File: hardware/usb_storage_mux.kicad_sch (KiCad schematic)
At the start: 25 parts, among them J8 Hirose USB3_B_Micro, J9 USB3_A, U6 TMUXHS4212

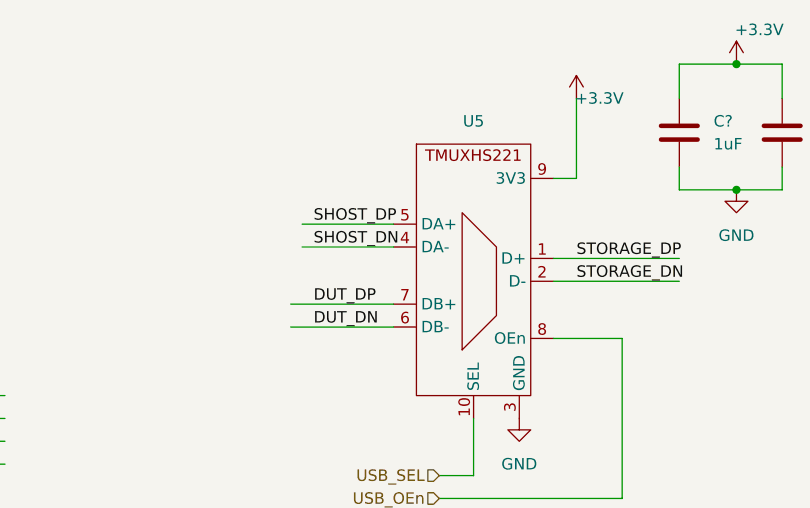
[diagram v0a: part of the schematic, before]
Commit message: Almost ready 2.0.0
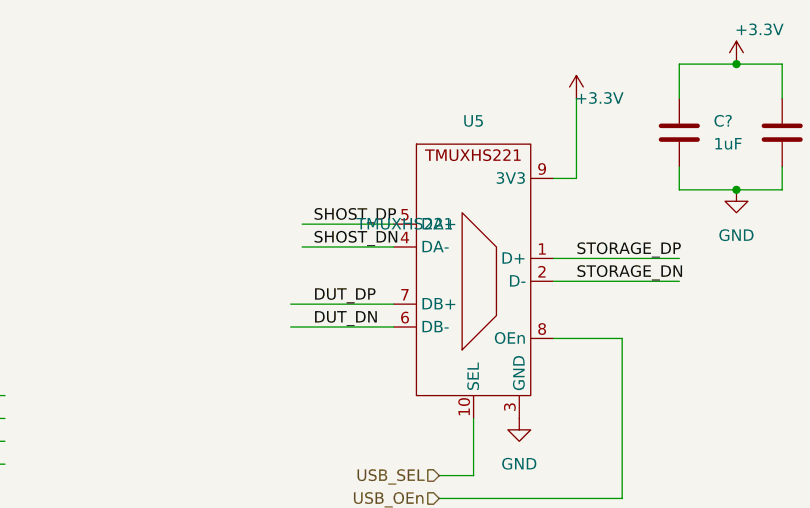
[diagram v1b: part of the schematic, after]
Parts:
- C25, C26, C27, C28, C? (x4): MFN (none) -> CL10B104KB8NNNC
- C? (x2): footprint Capacitor_SMD:C_0402_1005Metric -> Capacitor_SMD:C_0603_1608Metric; MFN (none) -> CL10B105KA8NNNC; MPN (none) -> CL10B105KA8NNNC
- C?: MFN (none) -> HV470M035E055ETR; MPN (none) -> HV470M035E055ETR
- D8: Link (none) -> https://www2.mouser.com/ProductDetail/onsemi-Fairchild/1N44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; MFN (none) -> 1N4448WT; MPN (none) -> 1N4448WT
- F2: MFN (none) -> MF-MSMF125-2; MPN (none) -> MF-MSMF125-2
- J8: Link https://www.mouser.es/c/connectors/usb-connectors/?product=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 -> https://www2.mouser.com/ProductDetail/Hirose-Connector/ZX36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; MFN (none) -> ZX360D-B-10P(30)
- J9: Link (none) -> https://eu.mouser.com/ProductDetail/Molex/48393-0001?qs=4Ef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; MFN (none) -> 48393-0001; MPN (none) -> 48393-0001
- Q? (x2): Link (none) -> https://www.mouser.es/ProductDetail/onsemi-Fairchild/FDC633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; MFN (none) -> FDC6330L; MPN (none) -> FDC6330L
- R? (x2): MFN (none) -> RTT024702FTH; MPN (none) -> RTT024702FTH
- R? (x2): MFN (none) -> RTT022201FTH; MPN (none) -> RTT022201FTH
- R? (x2): MFN (none) -> RTT02331JTH; MPN (none) -> RTT02331JTH
- U5: value ~ -> TMUXHS221; Link (none) -> https://eu.mouser.com/ProductDetail/Texas-Instruments/TMUXH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; MFN (none) -> TMUXHS221NKGR; MPN (none) -> TMUXHS221NKGR
- U6: Link (none) -> https://eu.mouser.com/ProductDetail/Texas-Instruments/TMUXH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; MFN (none) -> TMUXHS4212RKSR; MPN (none) -> TMUXHS4212RKSR
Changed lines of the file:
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@@
+      (effects (font (size 1.27 1.27)) hide)
+    )
+    (property "MFN" "RTT024702FTH" (at 195.58 85.09 0)
+      (effects (font (size 1.27 1.27)) hide)
+    )
+    (property "MPN" "RTT024702FTH" (at 195.58 85.09 0)
       (effects (font (size 1.27 1.27)) hide)
     )
@@
       (effects (font (size 1.27 1.27)) hide)
     )
+    (property "MFN" "CL10B104KB8NNNC" (at 163.83 113.03 0)
+      (effects (font (size 1.27 1.27)) hide)
+    )
     (pin "1")
     (pin "2")
@@
     )
     (property "Datasheet" "https://www.onsemi.com/pub/Collateral/FDC6330L-D.PDF" (at 207.01 90.17 0)
+      (effects (font (size 1.27 1.27)) hide)
+    )
+    (property "Link" "https://www.mouser.es/ProductDetail/onsemi-Fairchild/FDC6330L?qs=efMQ9B2bthfkfJJoj5%252B07g%3D%3D" (at 209.55 87.63 0)
+      (effects (font (size 1.27 1.27)) hide)
+    )
+    (property "MFN" "FDC6330L" (at 209.55 87.63 0)
+      (effects (font (size 1.27 1.27)) hide)
+    )
+    (property "MPN" "FDC6330L" (at 209.55 87.63 0)
       (effects (font (size 1.27 1.27)) hide)
     )
@@
       (effects (font (size 1.27 1.27)) hide)
     )
-    (property "Link" "https://www.mouser.es/c/connectors/usb-connectors/?product=Micro%20USB%20Type%20B%20Connectors&standard=USB%203.0&termination%20style=SMD%2FSMT&instock=y" (at 31.75 154.94 0)
+    (property "Link" "https://www2.mouser.com/ProductDetail/Hirose-Connector/ZX360D-B-10P30?qs=4J5DPWWS9EDezzYtx6NKEg%3D%3D" (at 31.75 154.94 0)
+      (effects (font (size 1.27 1.27)) hide)
+    )
+    (property "MFN" "ZX360D-B-10P(30)" (at 31.75 154.94 0)
       (effects (font (size 1.27 1.27)) hide)
     )
@@
       (effects (font (size 1.27 1.27)) hide)
     )
+    (property "MFN" "CL10B104KB8NNNC" (at 26.67 186.055 0)
+      (effects (font (size 1.27 1.27)) hide)
+    )
     (pin "1")
     (pin "2")
@@
       (effects (font (size 1.27 1.27)) (justify left))
     )
-    (property "Footprint" "Capacitor_SMD:C_0402_1005Metric" (at 158.4452 146.05 0)
+    (property "Footprint" "Capacitor_SMD:C_0603_1608Metric" (at 158.4452 146.05 0)
       (effects (font (size 1.27 1.27)) hide)
     )
@@
       (effects (font (size 1.27 1.27)) hide)
     )
+    (property "MFN" "CL10B105KA8NNNC" (at 157.48 142.24 0)
+      (effects (font (size 1.27 1.27)) hide)
+    )
+    (property "MPN" "CL10B105KA8NNNC" (at 157.48 142.24 0)
+      (effects (font (size 1.27 1.27)) hide)
+    )
     (pin "1")
     (pin "2")
@@
       (effects (font (size 1.27 1.27)) hide)
     )
+    (property "MFN" "RTT024702FTH" (at 194.31 40.64 0)
+      (effects (font (size 1.27 1.27)) hide)
+    )
+    (property "MPN" "RTT024702FTH" (at 194.31 40.64 0)
+      (effects (font (size 1.27 1.27)) hide)
+    )
     (pin "1")
     (pin "2")
@@
       (effects (font (size 1.27 1.27)) hide)
     )
+    (property "MFN" "RTT022201FTH" (at 208.28 57.15 0)
+      (effects (font (size 1.27 1.27)) hide)
+    )
+    (property "MPN" "RTT022201FTH" (at 208.28 57.15 0)
+      (effects (font (size 1.27 1.27)) hide)
+    )
     (pin "1")
     (pin "2")
@@
       (effects (font (size 1.27 1.27)) hide)
     )
+    (property "MFN" "CL10B104KB8NNNC" (at 91.44 121.92 0)
+      (effects (font (size 1.27 1.27)) hide)
+    )
     (pin "1")
     (pin "2")
@@
     )
     (property "Sim.Pins" "1=K 2=A" (at 269.24 71.755 0)
+      (effects (font (size 1.27 1.27)) hide)
+    )
+    (property "Link" "https://www2.mouser.com/ProductDetail/onsemi-Fairchild/1N4448WT?qs=2%2FYqgE%252BHg%252BJEFyXf7B7EGw%3D%3D" (at 269.24 71.755 0)
+      (effects (font (size 1.27 1.27)) hide)
+    )
+    (property "MFN" "1N4448WT" (at 269.24 71.755 0)
+      (effects (font (size 1.27 1.27)) hide)
+    )
+    (property "MPN" "1N4448WT" (at 269.24 71.755 0)
       (effects (font (size 1.27 1.27)) hide)
     )
@@
       (effects (font (size 1.27 1.27)) hide)
     )
+    (property "MFN" "CL10B104KB8NNNC" (at 168.91 142.24 0)
+      (effects (font (size 1.27 1.27)) hide)
+    )
     (pin "1")
     (pin "2")
@@
     )
     (property "Datasheet" "~" (at 259.08 140.335 0)
+      (effects (font (size 1.27 1.27)) hide)
+    )
+    (property "MFN" "RTT02331JTH" (at 259.08 140.335 0)
+      (effects (font (size 1.27 1.27)) hide)
+    )
+    (property "MPN" "RTT02331JTH" (at 259.08 140.335 0)
       (effects (font (size 1.27 1.27)) hide)
     )
@@
     )
     (property "Datasheet" "~" (at 256.54 105.41 0)
+      (effects (font (size 1.27 1.27)) hide)
+    )
+    (property "Link" "https://eu.mouser.com/ProductDetail/Molex/48393-0001?qs=4Ef8CTzXwRfUk7%252BJCOVflQ%3D%3D&_gl=1*l7r4pu*_ga*dW5kZWZpbmVk*_ga_15W4STQT4T*MTcwMjM3NTI2MC40MC4xLjE3MDIzNzUyNjEuNTkuMC4w" (at 260.35 107.95 0)
+      (effects (font (size 1.27 1.27)) hide)
+    )
+    (property "MFN" "48393-0001" (at 260.35 107.95 0)
+      (effects (font (size 1.27 1.27)) hide)
+    )
+    (property "MPN" "48393-0001" (at 260.35 107.95 0)
       (effects (font (size 1.27 1.27)) hide)
     )
@@
       (effects (font (size 1.27 1.27)) hide)
     )
+    (property "Description" "6V 1.25 A Resetable fuse" (at 242.57 87.63 0)
+      (effects (font (size 1.27 1.27)) hide)
+    )
+    (property "MFN" "MF-MSMF125-2" (at 242.57 87.63 0)
+      (effects (font (size 1.27 1.27)) hide)
+    )
+    (property "MPN" "MF-MSMF125-2" (at 242.57 87.63 0)
+      (effects (font (size 1.27 1.27)) hide)
+    )
     (pin "1")
     (pin "2")
@@
     )
     (property "Datasheet" "https://www.onsemi.com/pub/Collateral/FDC6330L-D.PDF" (at 205.74 45.72 0)
+      (effects (font (size 1.27 1.27)) hide)
+    )
+    (property "Link" "https://www.mouser.es/ProductDetail/onsemi-Fairchild/FDC6330L?qs=efMQ9B2bthfkfJJoj5%252B07g%3D%3D" (at 208.28 43.18 0)
+      (effects (font (size 1.27 1.27)) hide)
+    )
+    (property "MFN" "FDC6330L" (at 208.28 43.18 0)
+      (effects (font (size 1.27 1.27)) hide)
+    )
+    (property "MPN" "FDC6330L" (at 208.28 43.18 0)
       (effects (font (size 1.27 1.27)) hide)
     )
@@
       (effects (font (size 1.27 1.27)) hide)
     )
+    (property "MFN" "RTT02331JTH" (at 20.32 186.055 0)
+      (effects (font (size 1.27 1.27)) hide)
+    )
+    (property "MPN" "RTT02331JTH" (at 20.32 186.055 0)
+      (effects (font (size 1.27 1.27)) hide)
+    )
     (pin "1")
     (pin "2")
@@
       (effects (font (size 1.27 1.27)) (justify left))
     )
-    (property "Footprint" "Capacitor_SMD:C_0402_1005Metric" (at 127.9652 40.64 0)
+    (property "Footprint" "Capacitor_SMD:C_0603_1608Metric" (at 127.9652 40.64 0)
       (effects (font (size 1.27 1.27)) hide)
     )
@@
       (effects (font (size 1.27 1.27)) hide)
     )
+    (property "MFN" "CL10B105KA8NNNC" (at 127 36.83 0)
+      (effects (font (size 1.27 1.27)) hide)
+    )
+    (property "MPN" "CL10B105KA8NNNC" (at 127 36.83 0)
+      (effects (font (size 1.27 1.27)) hide)
+    )
     (pin "1")
     (pin "2")
@@
     )
     (property "MPN2" "TCC0402X7R104M160AT" (at 93.98 119.38 0)
+      (effects (font (size 1.27 1.27)) hide)
+    )
+    (property "MFN" "CL10B104KB8NNNC" (at 93.98 119.38 0)
       (effects (font (size 1.27 1.27)) hide)
     )
@@
     )
     (property "Datasheet" "https://www.ti.com/lit/ds/symlink/tmuxhs4212.pdf" (at 119.38 102.87 0)
+      (effects (font (size 1.27 1.27)) hide)
+    )
+    (property "Link" "https://eu.mouser.com/ProductDetail/Texas-Instruments/TMUXHS4212RKSR?qs=7MVldsJ5UawhO1PzGdCV7Q%3D%3" (at 119.38 102.87 0)
+      (effects (font (size 1.27 1.27)) hide)
+    )
+    (property "MFN" "TMUXHS4212RKSR" (at 119.38 102.87 0)
+      (effects (font (size 1.27 1.27)) hide)
+    )
+    (property "MPN" "TMUXHS4212RKSR" (at 119.38 102.87 0)
       (effects (font (size 1.27 1.27)) hide)
     )
@@
       (effects (font (size 1.27 1.27)) hide)
     )
+    (property "MFN" "CL10B104KB8NNNC" (at 161.29 115.57 0)
+      (effects (font (size 1.27 1.27)) hide)
+    )
     (pin "1")
     (pin "2")
@@
       (effects (font (size 1.27 1.27)) hide)
     )
+    (property "MFN" "CL10B104KB8NNNC" (at 138.43 36.83 0)
+      (effects (font (size 1.27 1.27)) hide)
+    )
     (pin "1")
     (pin "2")
@@
       (effects (font (size 1.27 1.27)) hide)
     )
+    (property "Description" "47uF 32V 6.3x5.4 SMD Electrolytic Capacitor" (at 226.06 83.82 0)
+      (effects (font (size 1.27 1.27)) hide)
+    )
+    (property "MFN" "HV470M035E055ETR" (at 226.06 83.82 0)
+      (effects (font (size 1.27 1.27)) hide)
+    )
+    (property "MPN" "HV470M035E055ETR" (at 226.06 83.82 0)
+      (effects (font (size 1.27 1.27)) hide)
+    )
     (pin "1")
     (pin "2")
@@
       (effects (font (size 1.27 1.27)))
     )
-    (property "Value" "~" (at 96.52 46.99 0)
+    (property "Value" "TMUXHS221" (at 96.52 46.99 0)
       (effects (font (size 1.27 1.27)))
     )
@@
     )
     (property "Datasheet" "https://www.ti.com/product/TMUXHS221" (at 96.52 46.99 0)
+      (effects (font (size 1.27 1.27)) hide)
+    )
+    (property "Link" "https://eu.mouser.com/ProductDetail/Texas-Instruments/TMUXHS221NKGR?qs=IPgv5n7u5QbuI%2Forjo3H9g%3D%3D" (at 96.52 46.99 0)
+      (effects (font (size 1.27 1.27)) hide)
+    )
+    (property "MFN" "TMUXHS221NKGR" (at 96.52 46.99 0)
+      (effects (font (size 1.27 1.27)) hide)
+    )
+    (property "MPN" "TMUXHS221NKGR" (at 96.52 46.99 0)
       (effects (font (size 1.27 1.27)) hide)
     )
@@
       (effects (font (size 1.27 1.27)) hide)
     )
+    (property "MFN" "RTT022201FTH" (at 209.55 101.6 0)
+      (effects (font (size 1.27 1.27)) hide)
+    )
+    (property "MPN" "RTT022201FTH" (at 209.55 101.6 0)
+      (effects (font (size 1.27 1.27)) hide)
+    )
     (pin "1")
     (pin "2")
@@
       (effects (font (size 1.27 1.27)) hide)
     )
+    (property "MFN" "CL10B104KB8NNNC" (at 265.43 140.335 0)
+      (effects (font (size 1.27 1.27)) hide)
+    )
